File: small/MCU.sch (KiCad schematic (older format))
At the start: 35 parts, among them IC1 PIC32MX350F256H-V_PT, J3 Micro_SD_Card, J4 Conn_01x05_Female, U5 AT25M02, U8 PCF8563T, Y2 Crystal

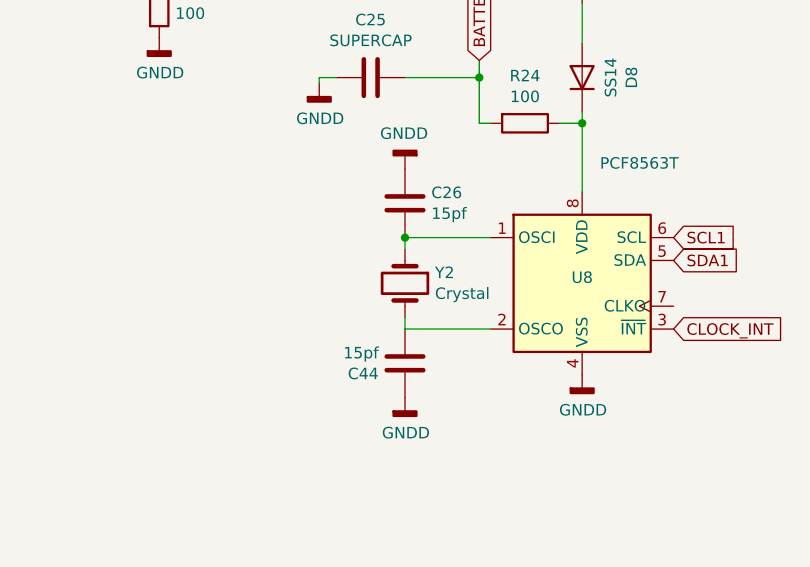
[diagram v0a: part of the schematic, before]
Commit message: BOM updated
Layout changed
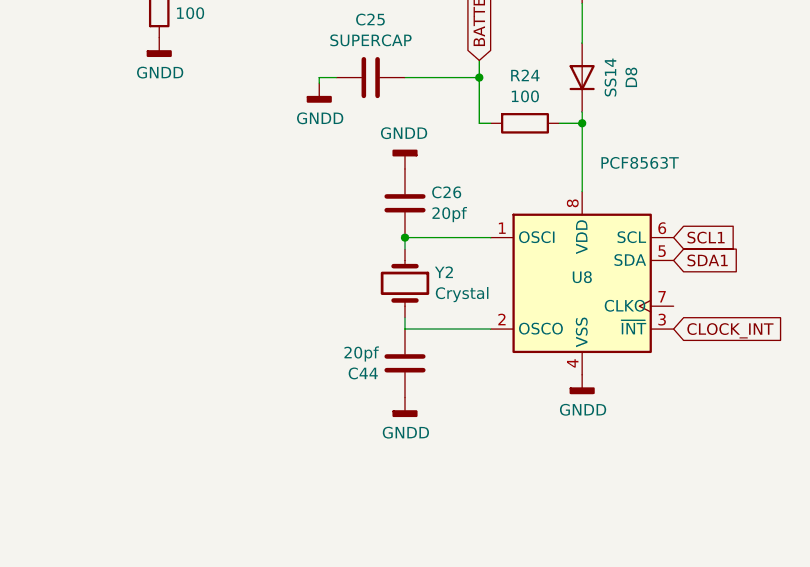
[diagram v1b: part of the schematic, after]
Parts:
- C15, C17, C18, C19, C20, C21, C24, C29, C30, C31: source (none) -> 0
- C25: source (none) -> 1
- C26, C44: value 15pf -> 20pf; MPN (none) -> CL10C200JB8NNNC; source (none) -> 0
- D10, D4: MPN (none) -> FC-2012HRK-620D; Price (none) -> 0.0199; source (none) -> 0
- D8: MPN (none) -> SS14; source (none) -> 0
- IC1: MPN (none) -> PIC32MX350F256H-V/PT; Manufacturer_Name Microchip -> (none); Manufacturer_Part_Number PIC32MX350F256H-V/PT -> (none)
- R24: MPN (none) -> 0603WAF1005T5E; Price (none) -> 0.0028; source (none) -> 0
- R39, R7: MPN (none) -> 0603WAF1000T5E; source (none) -> 0
- R5: MPN (none) -> 0603WAF1002T5E; source (none) -> 0
- R6: MPN (none) -> 0603WAF1001T5E; source (none) -> 0
- U5: Website (none) -> mouser; source (none) -> 0
- U8: MPN (none) -> PCF8563T; source (none) -> 0
- Y2: MPN (none) -> Q13FC1350000400; Price (none) -> 0.4291; source (none) -> 0
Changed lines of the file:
@@
 F 4 "C25804" H 1800 3350 50  0001 C CNN "LCSC"
 F 5 "0.02" H 1800 3350 50  0001 C CNN "Price"
+F 6 "0603WAF1002T5E" H 1800 3350 50  0001 C CNN "MPN"
+F 7 "0" H 1800 3350 50  0001 C CNN "source"
 	1    1800 3350
 	0    1    1    0
@@
 F 5 "0.0071" H 1075 3675 50  0001 C CNN "Price"
 F 6 "CC0603KRX7R9BB104" H 1075 3675 50  0001 C CNN "MPN"
+F 7 "0" H 1075 3675 50  0001 C CNN "source"
 	1    1075 3675
 	1    0    0    -1
@@
 F 4 " C21190" H 1800 3450 50  0001 C CNN "LCSC"
 F 5 "0.009" H 1800 3450 50  0001 C CNN "Price"
+F 6 "0603WAF1001T5E" H 1800 3450 50  0001 C CNN "MPN"
+F 7 "0" H 1800 3450 50  0001 C CNN "source"
 	1    1800 3450
 	0    1    1    0
@@
 F 3 "https://datasheet.lcsc.com/szlcsc/Foshan-NationStar-Optoelectronics-FC-2012HRK-620D_C84256.pdf" H 8125 3925 50  0001 C CNN
 F 4 "C84256" V 8125 3925 50  0001 C CNN "LCSC"
+F 5 "FC-2012HRK-620D" H 8125 3925 50  0001 C CNN "MPN"
+F 6 "0.0199" H 8125 3925 50  0001 C CNN "Price"
+F 7 "0" H 8125 3925 50  0001 C CNN "source"
 	1    8125 3925
 	0    -1   -1   0
@@
 F 4 "C22775" H 8125 4225 50  0001 C CNN "LCSC"
 F 5 "0.0019" H 8125 4225 50  0001 C CNN "Price"
+F 6 "0603WAF1000T5E" H 8125 4225 50  0001 C CNN "MPN"
+F 7 "0" H 8125 4225 50  0001 C CNN "source"
 	1    8125 4225
 	1    0    0    -1
@@
 F 4 "C7440" H 9975 5450 50  0001 C CNN "LCSC"
 F 5 "0.3876" H 9975 5450 50  0001 C CNN "Price"
+F 6 "PCF8563T" H 9975 5450 50  0001 C CNN "MPN"
+F 7 "0" H 9975 5450 50  0001 C CNN "source"
 	1    9975 5450
 	1    0    0    -1
@@
 AR Path="/6078415F/607D7927" Ref="C26"  Part="1"
 F 0 "C26" H 9315 5146 50  0000 L CNN
-F 1 "15pf" H 9315 5055 50  0000 L CNN
+F 1 "20pf" H 9315 5055 50  0000 L CNN
 F 2 "Capacitor_SMD:C_0603_1608Metric_Pad1.08x0.95mm_HandSolder" H 9238 4950 50  0001 C CNN
 F 3 "https://datasheet.lcsc.com/szlcsc/Samsung-Electro-Mechanics-CL10C150JB8NNNC_C1644.pdf" H 9200 5100 50  0001 C CNN
 F 4 "C1648" H 9200 5100 50  0001 C CNN "LCSC"
 F 5 "C1644" H 9200 5100 50  0001 C CNN "Price"
+F 6 "CL10C200JB8NNNC" H 9200 5100 50  0001 C CNN "MPN"
+F 7 "0" H 9200 5100 50  0001 C CNN "source"
 	1    9200 5100
 	1    0    0    -1
@@
 F 3 "https://datasheet.lcsc.com/szlcsc/1901081604_Seiko-Epson-Q13FC1350000400_C32346.pdf" H 9200 5450 50  0001 C CNN
 F 4 "C32346" V 9200 5450 50  0001 C CNN "LCSC"
+F 5 "Q13FC1350000400" H 9200 5450 50  0001 C CNN "MPN"
+F 6 "0.4291" H 9200 5450 50  0001 C CNN "Price"
+F 7 "0" H 9200 5450 50  0001 C CNN "source"
 	1    9200 5450
 	0    1    1    0
@@
 F 4 " C2480" H 9975 4550 50  0001 C CNN "LCSC"
 F 5 "0.0178" H 9975 4550 50  0001 C CNN "Price"
+F 6 "SS14" H 9975 4550 50  0001 C CNN "MPN"
+F 7 "0" H 9975 4550 50  0001 C CNN "source"
 	1    9975 4550
 	0    1    1    0
@@
 F 4 "KR-5R5C105-R" V 9050 4550 50  0001 C CNN "MPN"
 F 5 "C38065" H 9050 4550 50  0001 C CNN "LCSC"
+F 6 "1" H 9050 4550 50  0001 C CNN "source"
 	1    9050 4550
 	0    1    1    0
@@
 F 5 "AT25M02-SSHD-T" H 1650 7150 50  0001 C CNN "MPN"
 F 6 "2,60" H 1650 7150 50  0001 C CNN "Price"
+F 7 "mouser" H 1650 7150 50  0001 C CNN "Website"
+F 8 "0" H 1650 7150 50  0001 C CNN "source"
 	1    1650 7150
 	1    0    0    -1
@@
 F 3 "~" H 9725 4750 50  0001 C CNN
 F 4 " C7250" V 9725 4750 50  0001 C CNN "LCSC"
+F 5 "0603WAF1005T5E" H 9725 4750 50  0001 C CNN "MPN"
+F 6 "0.0028" H 9725 4750 50  0001 C CNN "Price"
+F 7 "0" H 9725 4750 50  0001 C CNN "source"
 	1    9725 4750
 	0    1    1    0
@@
 F 5 "0.0071" H 1075 2150 50  0001 C CNN "Price"
 F 6 "CC0603KRX7R9BB104" H 1075 2150 50  0001 C CNN "MPN"
+F 7 "0" H 1075 2150 50  0001 C CNN "source"
 	1    1075 2150
 	1    0    0    -1
@@
 F 5 "0.0071" H 1450 2150 50  0001 C CNN "Price"
 F 6 "CC0603KRX7R9BB104" H 1450 2150 50  0001 C CNN "MPN"
+F 7 "0" H 1450 2150 50  0001 C CNN "source"
 	1    1450 2150
 	1    0    0    -1
@@
 F 5 "0.0071" H 1825 2150 50  0001 C CNN "Price"
 F 6 "CC0603KRX7R9BB104" H 1825 2150 50  0001 C CNN "MPN"
+F 7 "0" H 1825 2150 50  0001 C CNN "source"
 	1    1825 2150
 	1    0    0    -1
@@
 F 5 "0.0071" H 2225 2150 50  0001 C CNN "Price"
 F 6 "CC0603KRX7R9BB104" H 2225 2150 50  0001 C CNN "MPN"
+F 7 "0" H 2225 2150 50  0001 C CNN "source"
 	1    2225 2150
 	1    0    0    -1
@@
 F 5 "0.0071" H 2600 2150 50  0001 C CNN "Price"
 F 6 "CC0603KRX7R9BB104" H 2600 2150 50  0001 C CNN "MPN"
+F 7 "0" H 2600 2150 50  0001 C CNN "source"
 	1    2600 2150
 	1    0    0    -1
@@
 F 5 "0.0071" H 8400 2800 50  0001 C CNN "Price"
 F 6 "CC0603KRX7R9BB104" H 8400 2800 50  0001 C CNN "MPN"
+F 7 "0" H 8400 2800 50  0001 C CNN "source"
 	1    8400 2800
 	1    0    0    -1
@@
 F 5 "TAJA106K016RNJ" H 5050 725 50  0001 C CNN "MPN"
 F 6 "0.2135" H 5050 725 50  0001 C CNN "Price"
+F 7 "0" H 5050 725 50  0001 C CNN "source"
 	1    5050 725
 	0    1    1    0
@@
 F 5 "0.0071" H 2125 3775 50  0001 C CNN "Price"
 F 6 "CC0603KRX7R9BB104" H 2125 3775 50  0001 C CNN "MPN"
+F 7 "0" H 2125 3775 50  0001 C CNN "source"
 	1    2125 3775
 	1    0    0    -1
@@
 F 5 "0.0071" H 2775 7150 50  0001 C CNN "Price"
 F 6 "CC0603KRX7R9BB104" H 2775 7150 50  0001 C CNN "MPN"
+F 7 "0" H 2775 7150 50  0001 C CNN "source"
 	1    2775 7150
 	1    0    0    -1
@@
 AR Path="/6078415F/609E1851" Ref="C44"  Part="1"
 F 0 "C44" H 9315 5846 50  0000 L CNN
-F 1 "15pf" H 9315 5755 50  0000 L CNN
+F 1 "20pf" H 9315 5755 50  0000 L CNN
 F 2 "Capacitor_SMD:C_0603_1608Metric_Pad1.08x0.95mm_HandSolder" H 9238 5650 50  0001 C CNN
 F 3 "https://datasheet.lcsc.com/szlcsc/Samsung-Electro-Mechanics-CL10C150JB8NNNC_C1644.pdf" H 9200 5800 50  0001 C CNN
 F 4 "C1648" H 9200 5800 50  0001 C CNN "LCSC"
 F 5 "C1644" H 9200 5800 50  0001 C CNN "Price"
+F 6 "CL10C200JB8NNNC" H 9200 5800 50  0001 C CNN "MPN"
+F 7 "0" H 9200 5800 50  0001 C CNN "source"
 	1    9200 5800
 	-1   0    0    1
@@
 F 3 "https://datasheet.lcsc.com/szlcsc/Foshan-NationStar-Optoelectronics-FC-2012HRK-620D_C84256.pdf" H 6200 875 50  0001 C CNN
 F 4 "C84256" V 6200 875 50  0001 C CNN "LCSC"
+F 5 "FC-2012HRK-620D" H 6200 875 50  0001 C CNN "MPN"
+F 6 "0.0199" H 6200 875 50  0001 C CNN "Price"
+F 7 "0" H 6200 875 50  0001 C CNN "source"
 	1    6200 875
 	-1   0    0    1
@@
 F 4 "C22775" H 6500 875 50  0001 C CNN "LCSC"
 F 5 "0.0019" H 6500 875 50  0001 C CNN "Price"
+F 6 "0603WAF1000T5E" H 6500 875 50  0001 C CNN "MPN"
+F 7 "0" H 6500 875 50  0001 C CNN "source"
 	1    6500 875
 	0    -1   -1   0
@@
 F 4 "Microchip PIC32MX350F256H-V/PT, 32bit PIC Microcontroller, 100MHz, 256 kB Flash, 64-Pin TQFP" H 6950 3850 50  0001 L CNN "Description"
 F 5 "1.2" H 6950 3750 50  0001 L CNN "Height"
-F 6 "Microchip" H 6950 3650 50  0001 L CNN "Manufacturer_Name"
-F 7 "PIC32MX350F256H-V/PT" H 6950 3550 50  0001 L CNN "Manufacturer_Part_Number"
+F 6 "" H 6950 3650 50  0001 L CNN "Manufacturer_Name"
+F 7 "" H 6950 3550 50  0001 L CNN "Manufacturer_Part_Number"
 F 8 "579-32MX350F256HVPT" H 6950 3450 50  0001 L CNN "Mouser Part Number"
 F 9 "https://www.mouser.com/Search/Refine.aspx?Keyword=579-32MX350F256HVPT" H 6950 3350 50  0001 L CNN "Mouser Price/Stock"
 F 10 "PIC32MX350F256H-V/PT" H 6950 3250 50  0001 L CNN "Arrow Part Number"
 F 11 "https://www.arrow.com/en/products/pic32mx350f256h-vpt/microchip-technology" H 6950 3150 50  0001 L CNN "Arrow Price/Stock"
+F 12 "PIC32MX350F256H-V/PT" H 3400 2850 50  0001 C CNN "MPN"
 	1    3400 2850
 	1    0    0    -1
